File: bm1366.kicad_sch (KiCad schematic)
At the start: 7 parts, among them J2 Conn_01x06, U35 TXU0304PW, U8 25MHz

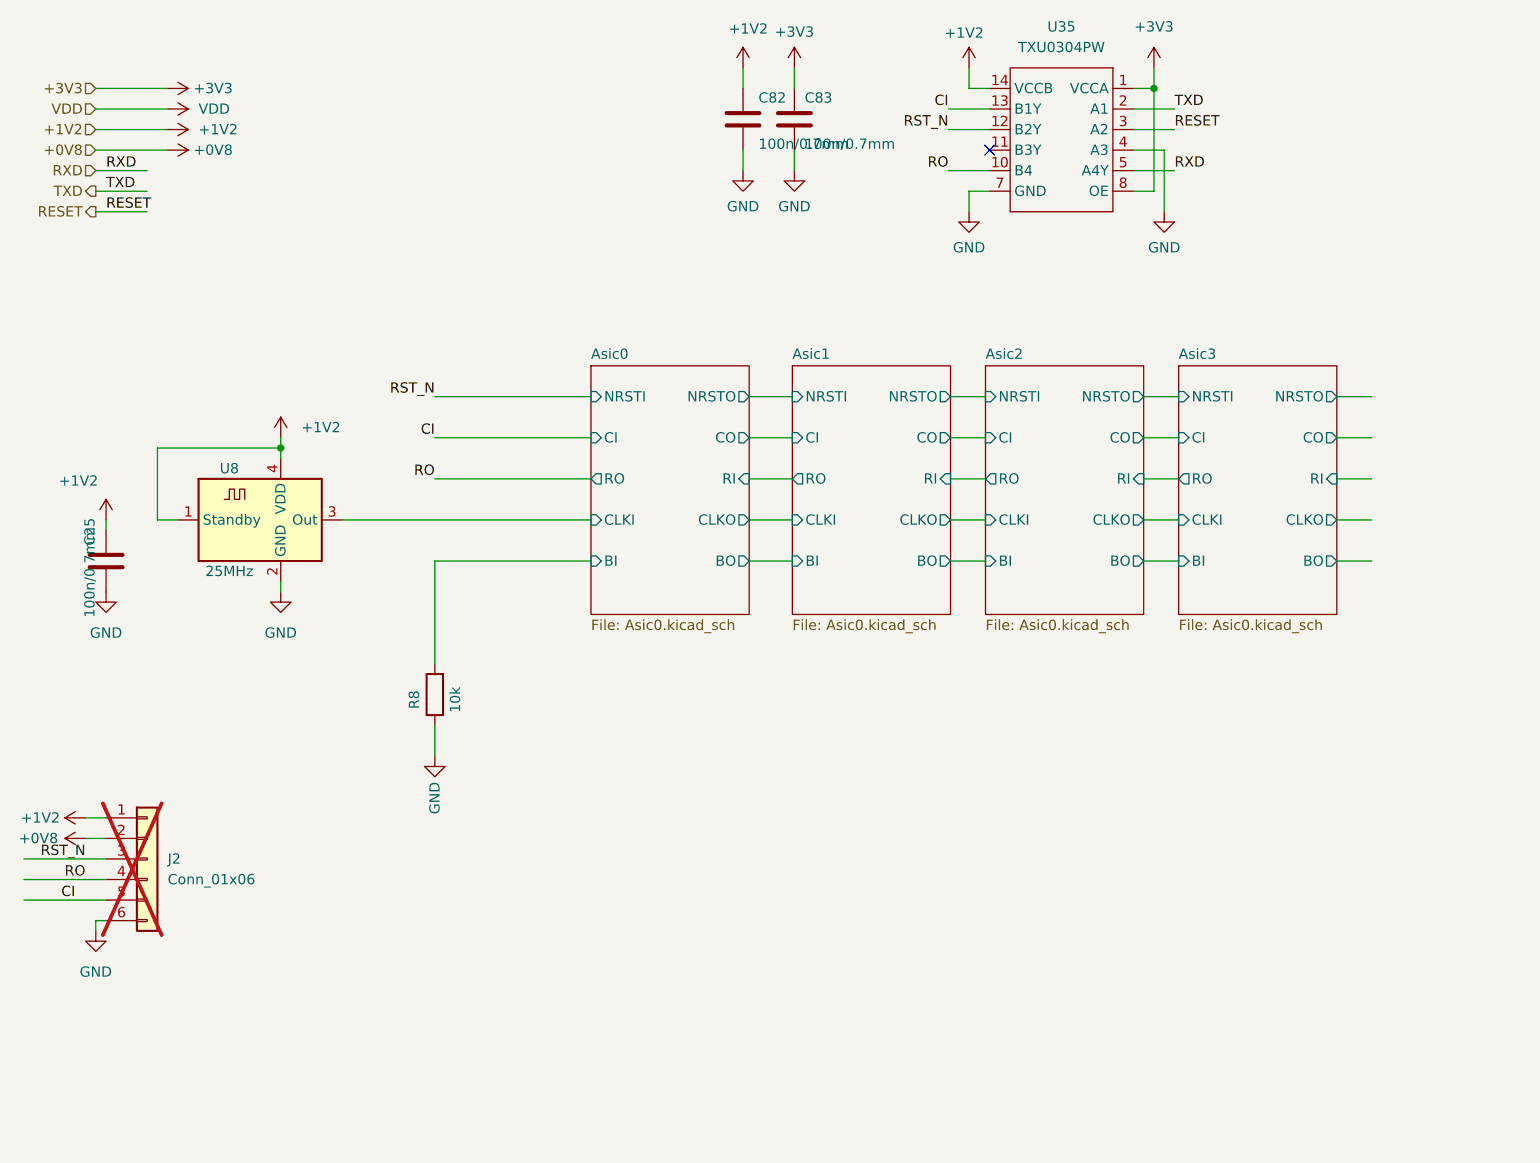
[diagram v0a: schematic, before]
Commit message: power stage in place
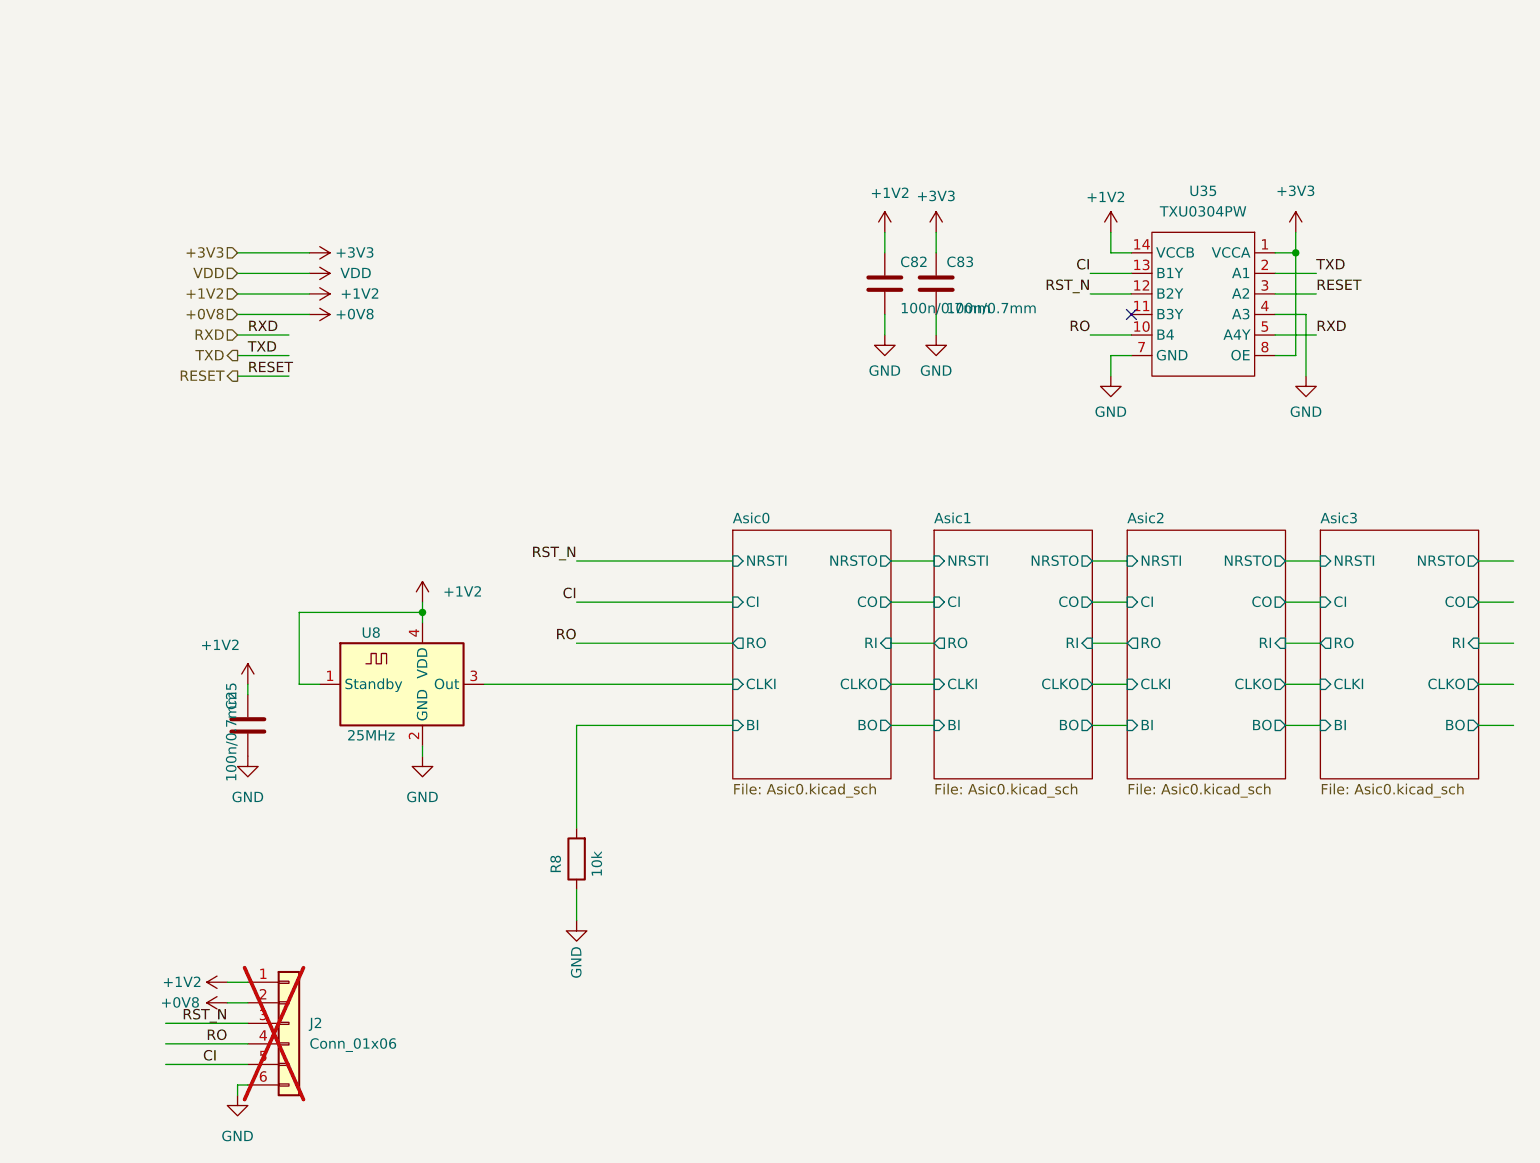
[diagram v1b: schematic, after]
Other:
- moved on the sheet: C25, C82, C83, J2, R8, U35, U8

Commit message: Add LCSC number to components
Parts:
- C25, C82, C83: LCSC (none) -> C694249
- R8: LCSC (none) -> C84376
- U35: LCSC (none) -> C4364118
- U8: LCSC (none) -> C9006
